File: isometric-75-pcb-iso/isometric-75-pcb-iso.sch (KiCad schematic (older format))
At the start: 11 parts, among them J1 Conn_01x05, SW1 SW_Push, U1 STM32F072CBTx

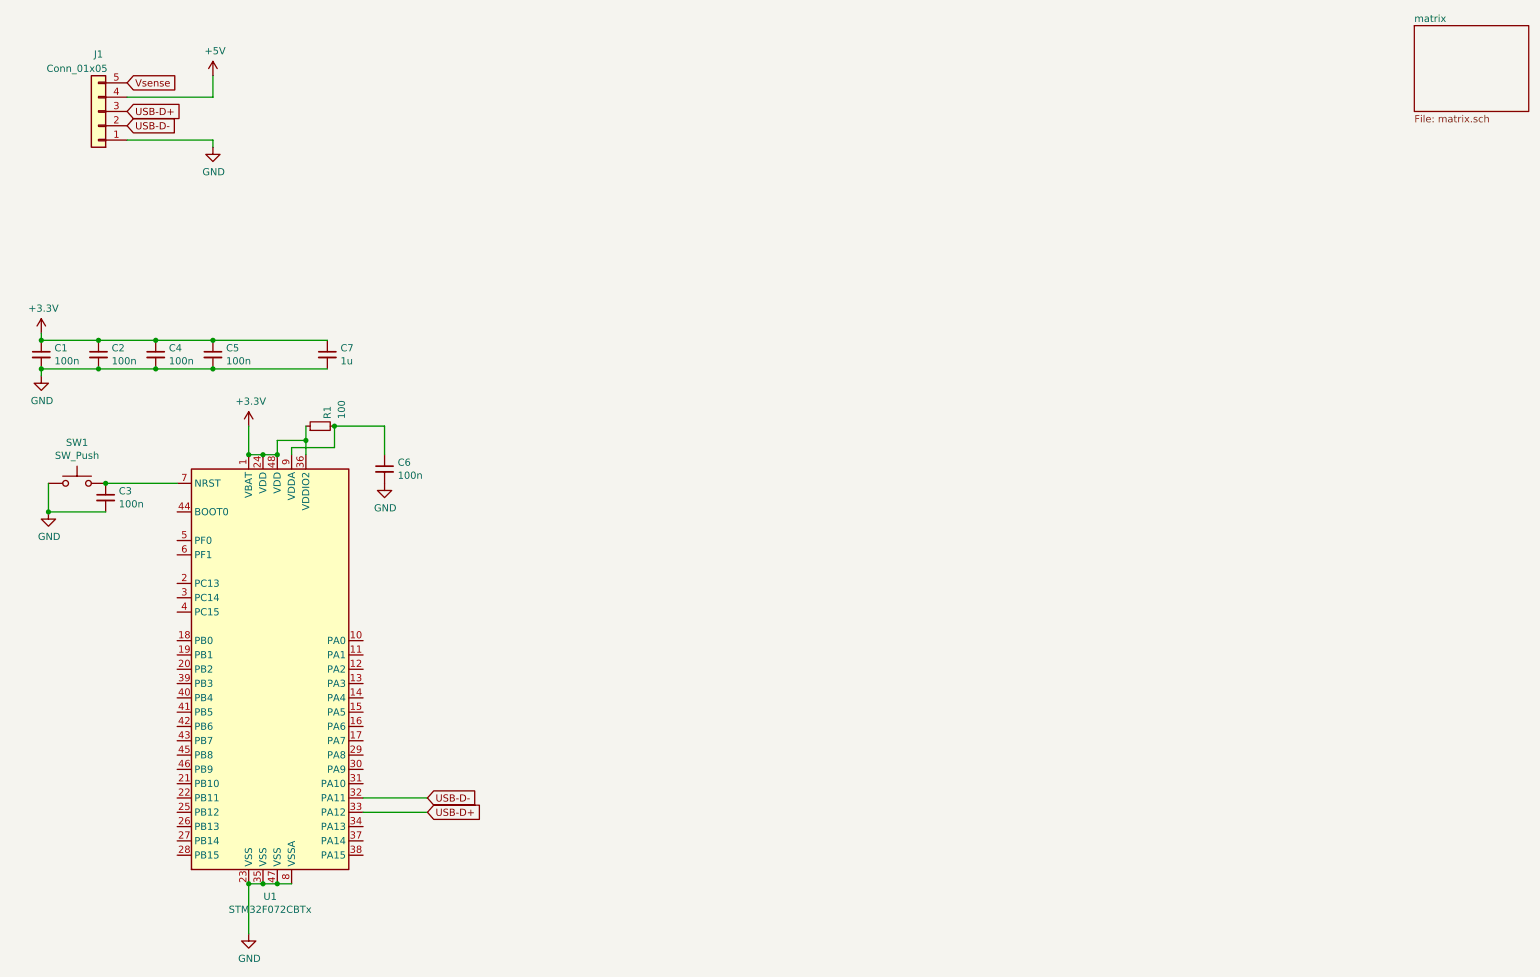
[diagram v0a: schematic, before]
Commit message: continued the pcb
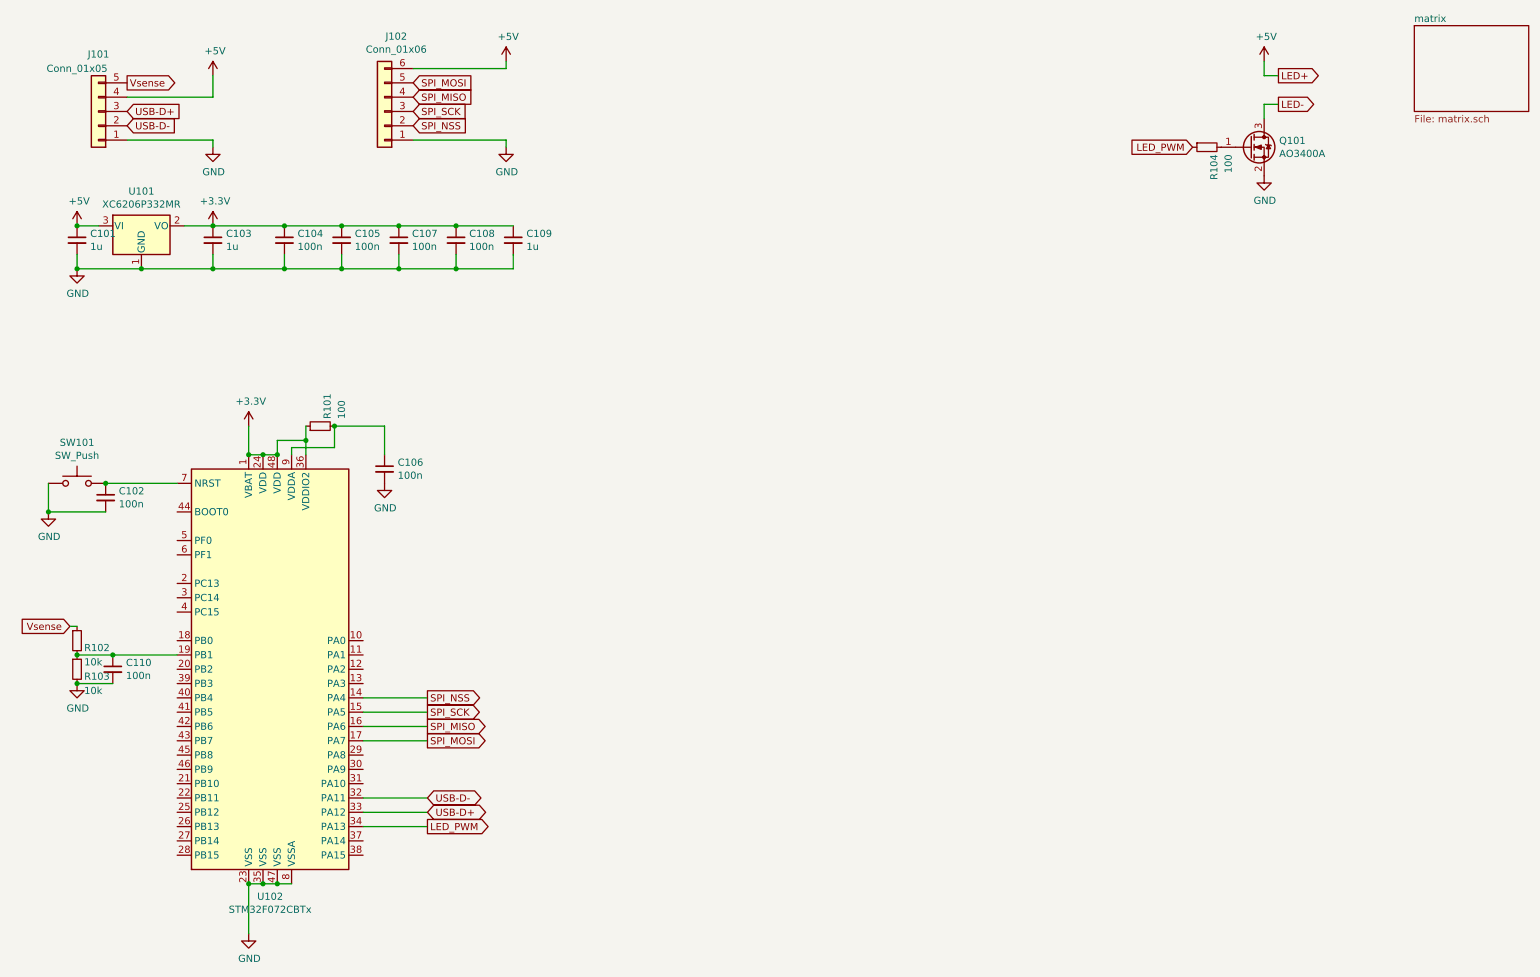
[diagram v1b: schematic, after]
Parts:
- added C101, C103: 1u, Capacitor_SMD:C_0402_1005Metric, symbol Device:C_Small
- added C110: 100n, Capacitor_SMD:C_0402_1005Metric, symbol Device:C_Small
- added J102: Conn_01x06, Connector_JST:JST_SH_SM06B-SRSS-TB_1x06-1MP_P1.00mm_Horizontal, symbol Connector_Generic:Conn_01x06
- added Q101: AO3400A, Package_TO_SOT_SMD:SOT-23, symbol Device:Q_NMOS_GSD
- added R102, R103: 10k, Resistor_SMD:R_0402_1005Metric, symbol Device:R_Small
- added R104: 100, Resistor_SMD:R_0402_1005Metric, symbol Device:R_Small
- added U101: XC6206P332MR, Package_TO_SOT_SMD:SOT-23, symbol Regulator_Linear:XC6206PxxxMR
- renumbered C3 to C102, C1 to C104, C2 to C105, C6 to C106, C4 to C107, C5 to C108, C7 to C109, J1 to J101, R1 to R101, SW1 to SW101, U1 to U102
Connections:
- net +3V3: now also C103.1, U101.2 (VO)
- net +5V: now also C101.1, J102.6 (Pin_6), U101.3 (VI)
- net GND: now also C101.2, C103.2, C110.2, J102.1 (Pin_1), Q101.2 (S), R103.2, U101.1 (GND)
- net Vsense: now also R102.1
- net SPI_NSS: now reaches U102.14 (PA4)
- net SPI_NSS: now also J102.2 (Pin_2)
- net SPI_SCK: now reaches U102.15 (PA5)
- net SPI_SCK: now also J102.3 (Pin_3)
- net SPI_MISO: now reaches U102.16 (PA6)
- net SPI_MISO: now also J102.4 (Pin_4)
- net SPI_MOSI: now reaches U102.17 (PA7)
- net SPI_MOSI: now also J102.5 (Pin_5)
- net at U102.19 (PB1): now also C110.1, R102.2, R103.1
- net LED_PWM: now reaches U102.34 (PA13)
- net LED_PWM: now also R104.1
- new net: Q101.1 (G), R104.2
- new net LED-: Q101.3 (D)
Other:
- moved on the sheet: C104, C105, C107, C108, C109
